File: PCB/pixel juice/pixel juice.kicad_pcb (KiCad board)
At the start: 2 copper layers, 99.7 x 52.4 mm, 18 parts, among them J1 n8 Bus Connector, J2 IRQ_SEL, J3 AUDIO_CLK, J4 PJRAN3X1U03X, J5 TO_AMP, J6 FROM_AMP, U1 TMS9128, U2 TMS4416, U3 TMS4416, U4 74LS32, Y1 10.738635Mhz

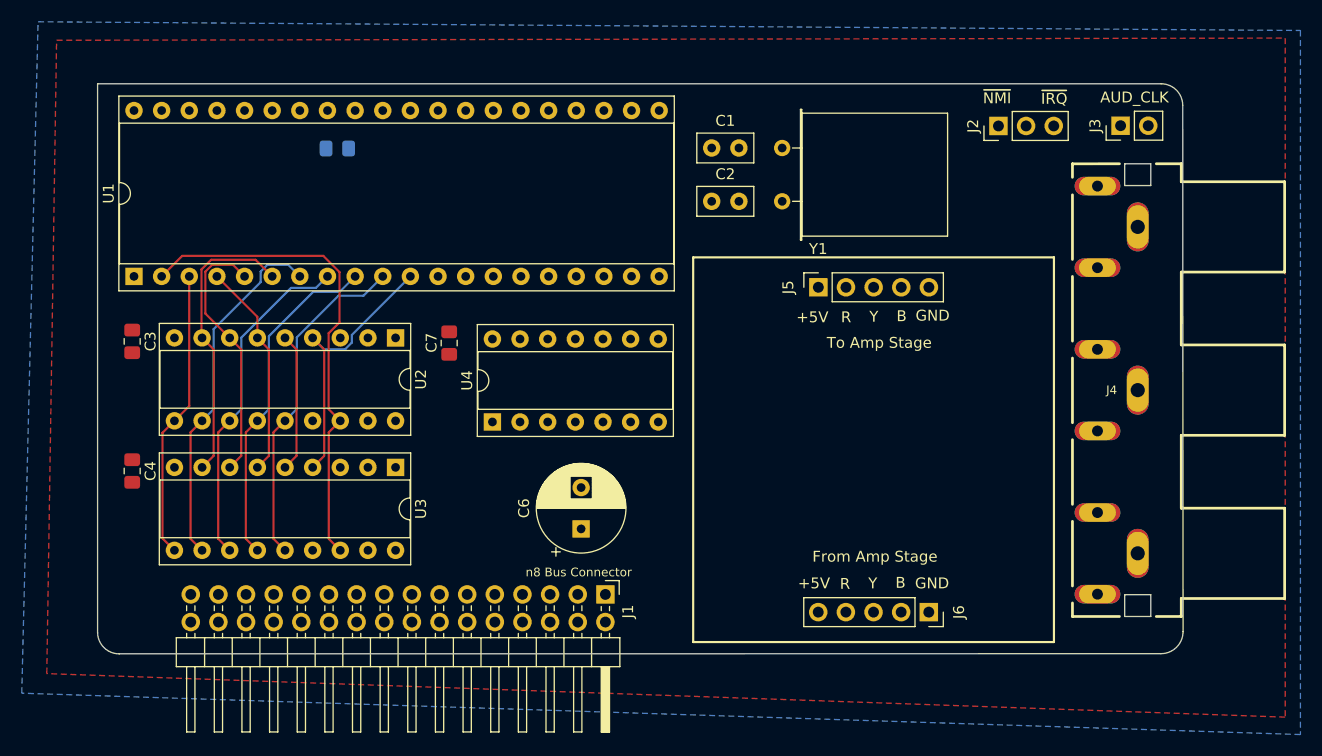
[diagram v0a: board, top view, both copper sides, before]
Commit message: rc1 before library swap test
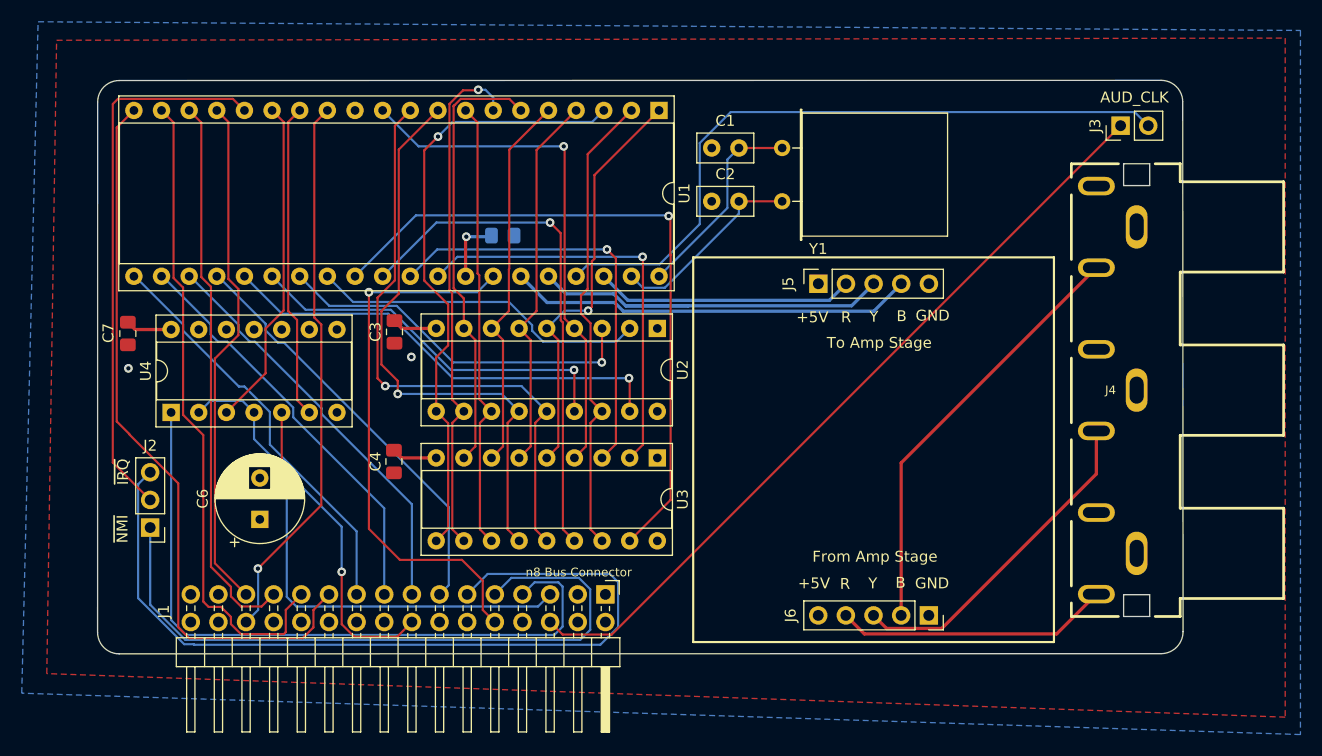
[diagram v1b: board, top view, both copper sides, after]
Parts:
- moved J2 86.2 mm to (105.4, 106.4), turned to 180 degrees
- moved U1 50.6 mm to (152.2, 68.0), turned to -90 degrees
- moved C6 29.5 mm to (115.5, 105.6)
- moved C7 29.5 mm to (103.3, 88.5)
- moved U4 29.5 mm to (107.3, 95.8)
- moved C3 24.1 mm to (127.8, 88.4)
- moved C4 24.1 mm to (127.8, 100.3)
- moved U2 24.1 mm to (152.0, 88.1)
- moved U3 24.1 mm to (152.0, 100.0)
- moved C5 17.2 mm to (137.8, 79.5)
- moved J5 0.33 mm to (166.8, 84.0)
- moved J6 0.30 mm to (176.9, 114.5)
- moved J4 0.10 mm to (193.7, 93.8)
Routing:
- net ~{IRQ}: track 0.00 -> 77.7 mm
- net AUDIO_CLK_{OUT}: track 0.00 -> 72.3 mm
- net D3: track 0.00 -> 67.4 mm
- net ~{READ}: track 0.00 -> 63.9 mm
- net AUDIO_CLK_{IN}: track 0.00 -> 63.7 mm
- net ~{NMI}: track 0.00 -> 62.8 mm
- net RD3: track 0.00 -> 62.6 mm, vias 0 -> 1
- net D2: track 0.00 -> 60.1 mm
- net D1: track 0.00 -> 51.0 mm
- net A0: track 0.00 -> 50.7 mm, vias 0 -> 1
- net ~{INT}: track 0.00 -> 50.5 mm
- net ~{RES}: track 0.00 -> 50.5 mm, vias 0 -> 1
- net RD2: track 0.00 -> 47.6 mm, vias 0 -> 1
- net D0: track 0.00 -> 47.4 mm
- net ~{WRITE}: track 0.00 -> 42.2 mm, vias 0 -> 1
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- added copper zone on In2.Cu, net +5V
- added copper zone on In1.Cu, net GND
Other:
- board size 99.7 x 52.4 mm -> 99.7 x 52.7 mm
- copper layers 2 -> 4
- board text added: "Pixel Juice v1.0b, April 2023 by Nate Rivard"
